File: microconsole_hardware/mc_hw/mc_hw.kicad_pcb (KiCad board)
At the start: 2 copper layers, 25 parts, among them SW1 DPAD - UP, SW10 START, SW11 L1, SW12 R1, SW13 L2, SW14 R2, SW16 Joystick, SW17 Joystick, SW2 DPAD - DOWN, SW3 DPAD - LEFT, SW4 DPAD - RIGHT, SW5 A, SW6 B, SW7 X, SW8 Y, SW9 SELECT, U1 CR2013-MI2120, U2 MAX98357A, U3 MCP23017x-x-SO

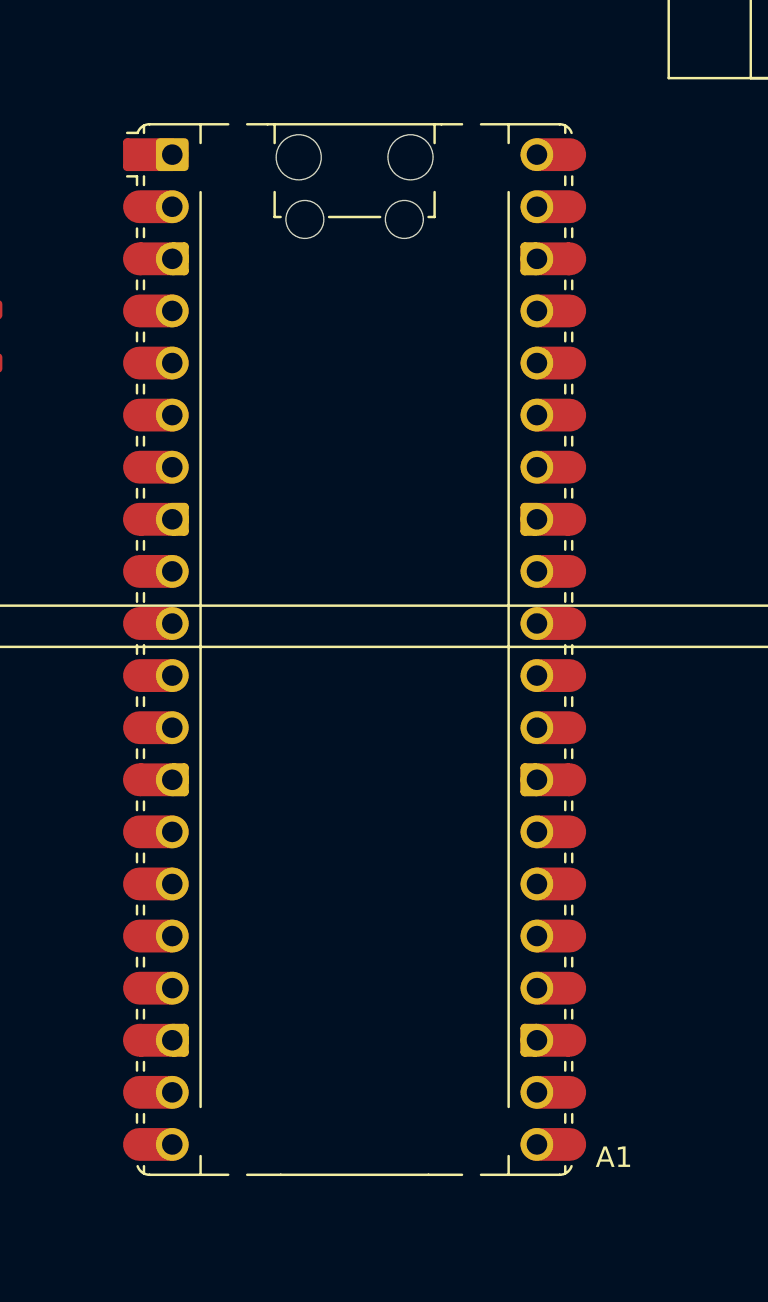
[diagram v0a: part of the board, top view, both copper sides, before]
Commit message: quick fix
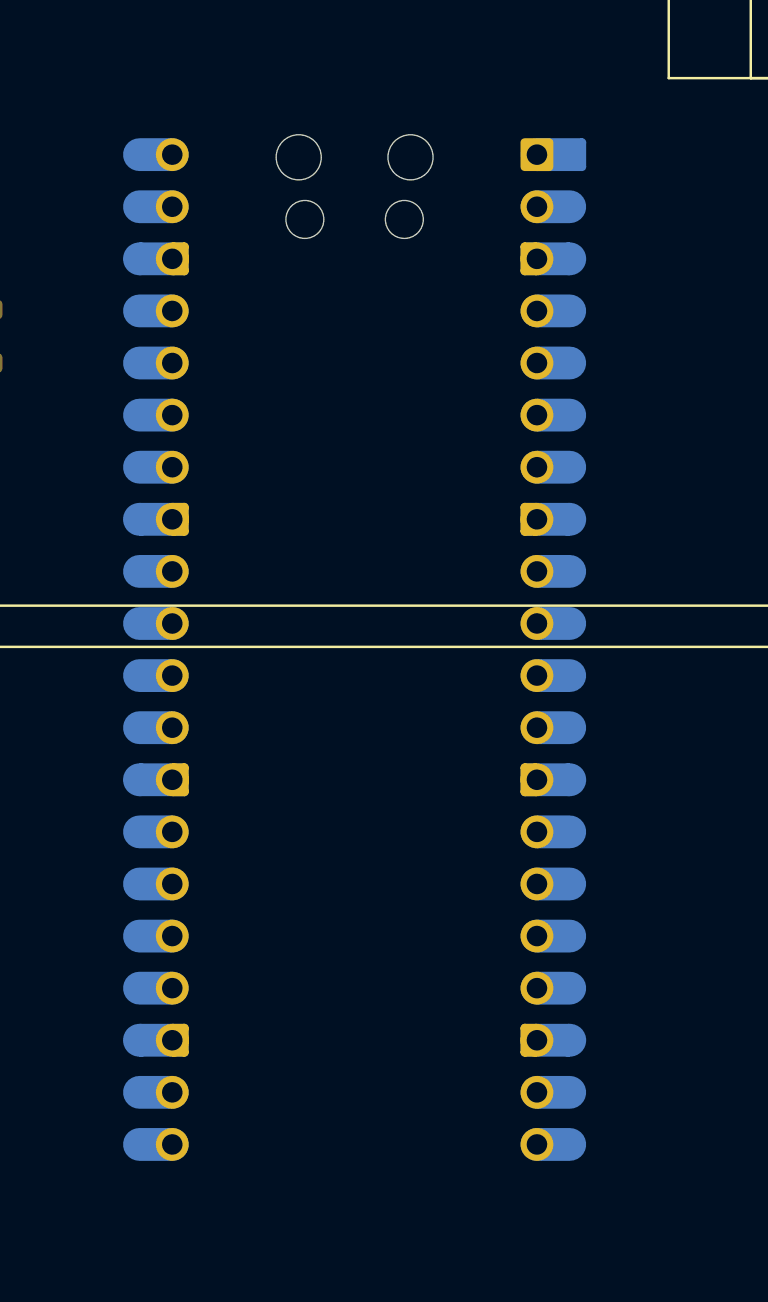
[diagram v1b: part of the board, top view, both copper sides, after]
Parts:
- A1: moved to B.Cu
- turned A1 to 180 degrees
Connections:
- net GPIO3 / MCP|ADC SCK renamed GPIO3 / MCP|ADC SCL
- net GPIO4 / ILI MISO renamed GPIO4 / LCD MISO
- net GPIO5 / ILI CS renamed GPIO5 / LCD CS
- net GPIO6 / ILI SCK renamed GPIO6 / LCD SCK
- net GPIO7 / ILI MOSI renamed GPIO7 / LCD MOSI
- net GPIO8 / ILI RESET renamed GPIO8 / LCD RESET
- net GPIO9 / ILI DC renamed GPIO9 / LCD DC
- U3 pad 9: VBUS -> 3v3
